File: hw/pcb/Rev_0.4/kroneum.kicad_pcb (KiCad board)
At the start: 2 copper layers, 43.7 x 40 mm, 23 parts, among them J1 USB_B_Micro, SW1 Boot_Mode_Btn, SW2 Ctrl_One_Btn, SW3 Reset_Btn, SW4 Ctrl_Ten_Btn, U1 STM32F042F4Px, U2 MCP1700-3302E_SOT89

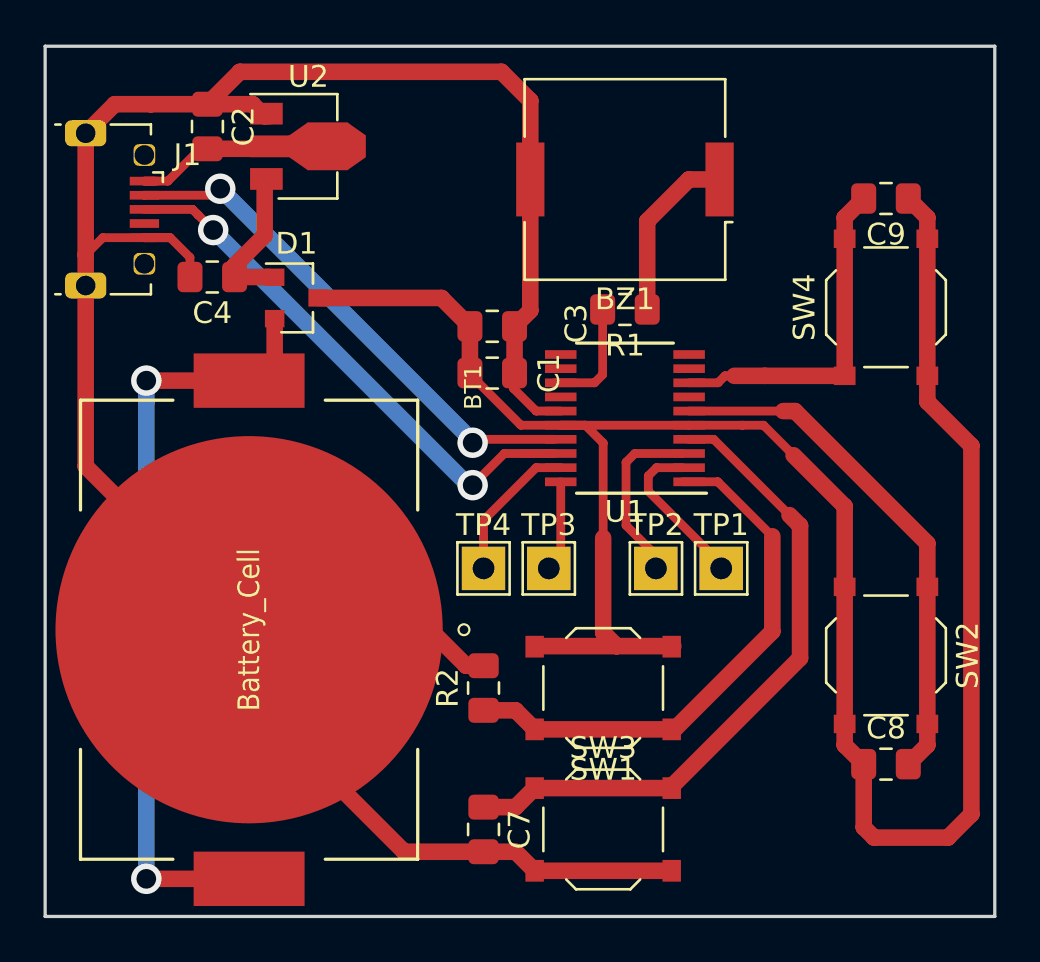
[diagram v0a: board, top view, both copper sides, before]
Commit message: hw: finish Rev 0.4 PCB layout.
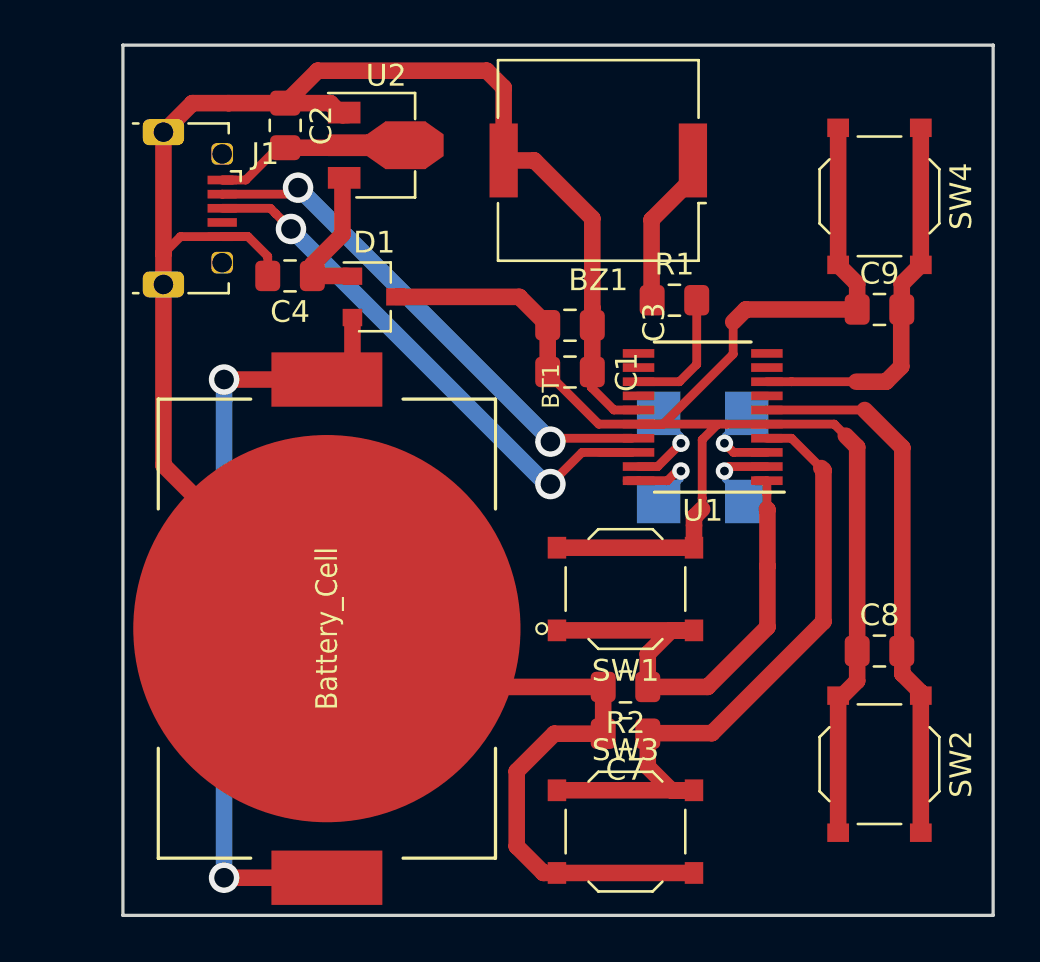
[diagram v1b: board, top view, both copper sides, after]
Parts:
- SW1: value Boot_Mode_Btn -> Boot
- SW2: value Ctrl_One_Btn -> One
- SW3: value Reset_Btn -> Reset
- SW4: value Ctrl_Ten_Btn -> Ten
- TP1, TP2, TP3, TP4: moved to B.Cu
- moved TP4 10.8 mm to (149.6, 109.9), turned to 180 degrees
- moved TP2 8.26 mm to (153.6, 109.9), turned to 180 degrees
- moved C7 7.87 mm to (148.0, 124.6), turned to 180 degrees
- moved R2 6.53 mm to (148.0, 122.5), turned to 180 degrees
- moved TP3 5.91 mm to (149.6, 113.9), turned to 180 degrees
- moved C8 5.21 mm to (159.7, 120.8)
- moved C9 5.11 mm to (159.7, 105.1), turned to 0 degrees
- moved SW4 5.11 mm to (159.7, 99.9), turned to 270 degrees
- moved SW2 5.01 mm to (159.7, 126.0)
- moved SW1 4.66 mm to (148.0, 118.0)
- moved BT1 3.58 mm to (134.3, 119.8)
- moved J1 3.58 mm to (128.0, 100.5)
- moved C1 3.58 mm to (145.5, 108.0)
- moved C2 3.58 mm to (132.4, 96.6)
- moved C3 3.58 mm to (145.5, 105.8)
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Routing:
- net VDD: track 103.7 -> 77.4 mm
- net GND: track 112.6 -> 120.2 mm
- net SCL: track 8.21 -> 3.92 mm, vias 0 -> 1
- net SDA: track 7.92 -> 3.86 mm, vias 0 -> 1
- net SWDIO: track 6.76 -> 4.19 mm, vias 0 -> 1
- net Ctrl_Ten: track 15.8 -> 18.0 mm
- net Net-(BZ1-Pad1): track 8.18 -> 7.22 mm
- net Ctrl_One: track 24.0 -> 24.8 mm
- net BOOT0: track 25.1 -> 24.3 mm
- net Buzzer: track 5.38 -> 5.95 mm
- net SWCLK: track 4.21 -> 4.31 mm, vias 0 -> 1
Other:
- board size 43.7 x 40 mm -> 40 x 40 mm
